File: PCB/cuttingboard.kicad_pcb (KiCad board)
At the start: 2 copper layers, 21 x 51 mm, 43 parts, among them J1 USB_C_Receptacle_USB2.0_14P, J2 Conn_01x20, J3 Conn_01x20, J4 Conn_01x03, SW1 SW_Push, U1 RP2040, U2 MPU-6050, U3 W25Q128JVS, U4 MCP1700x-330xxTT, Y1 12 MHz

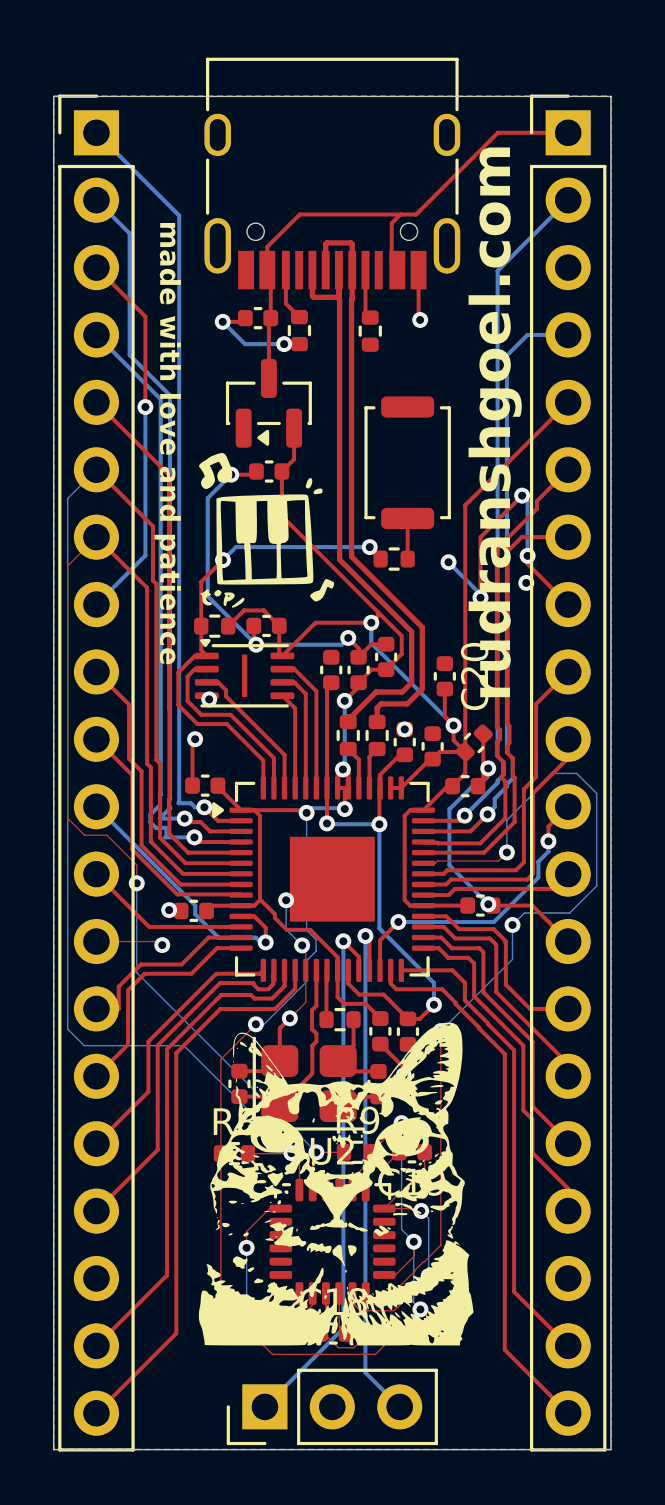
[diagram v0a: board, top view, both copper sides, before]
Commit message: added firmware and updated pcb files
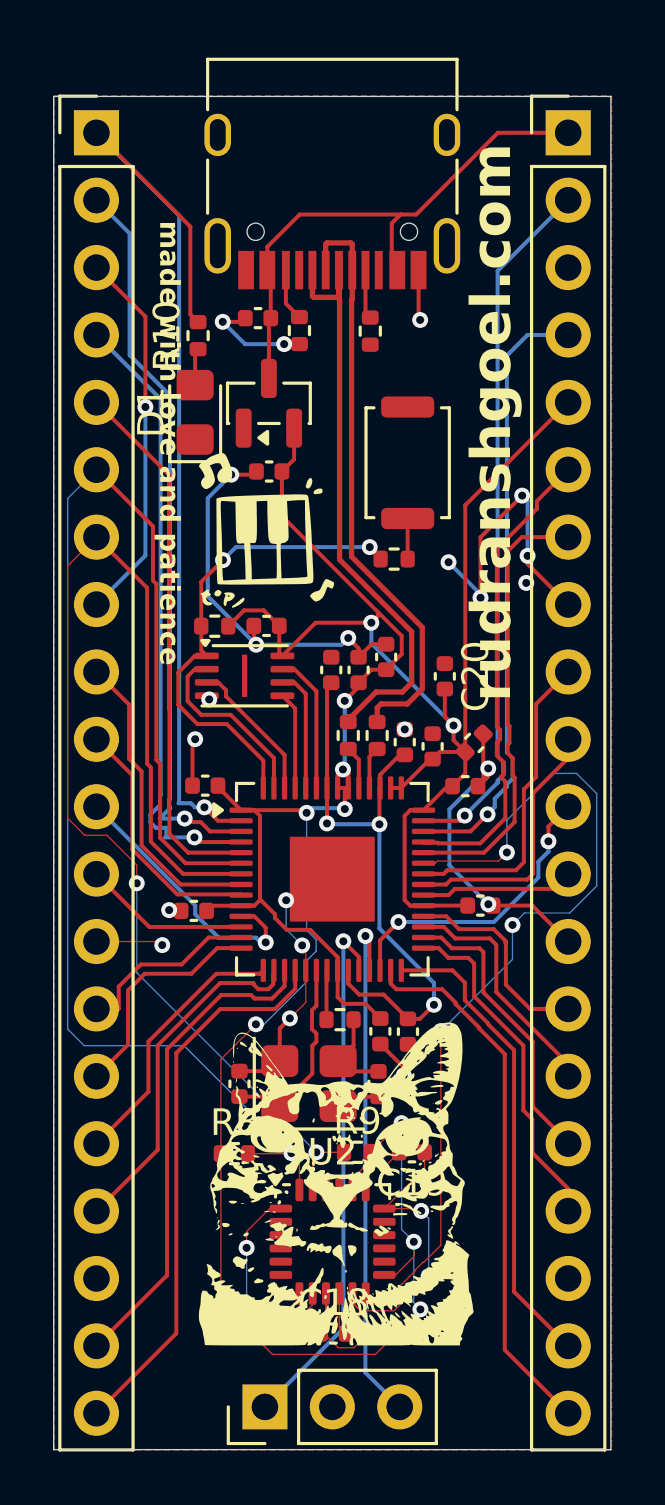
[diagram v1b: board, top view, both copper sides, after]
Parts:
- added D1: LED, LED_SMD:LED_0805_2012Metric_Pad1.15x1.40mm_HandSolder, F.Cu at (97.1, 69.7)
- added R10: 1K, Resistor_SMD:R_0402_1005Metric, F.Cu at (97.2, 66.8)
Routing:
- net GPIO0: track 29.2 -> 37.9 mm
- net Net-(D1-A): track 0.00 -> 1.40 mm
